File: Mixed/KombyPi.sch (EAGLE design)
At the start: 15 parts, among them IC3 DS1307, J1 POWER_JACKPTH, J2 MOLEX-39501XXX4, Q1 32.768

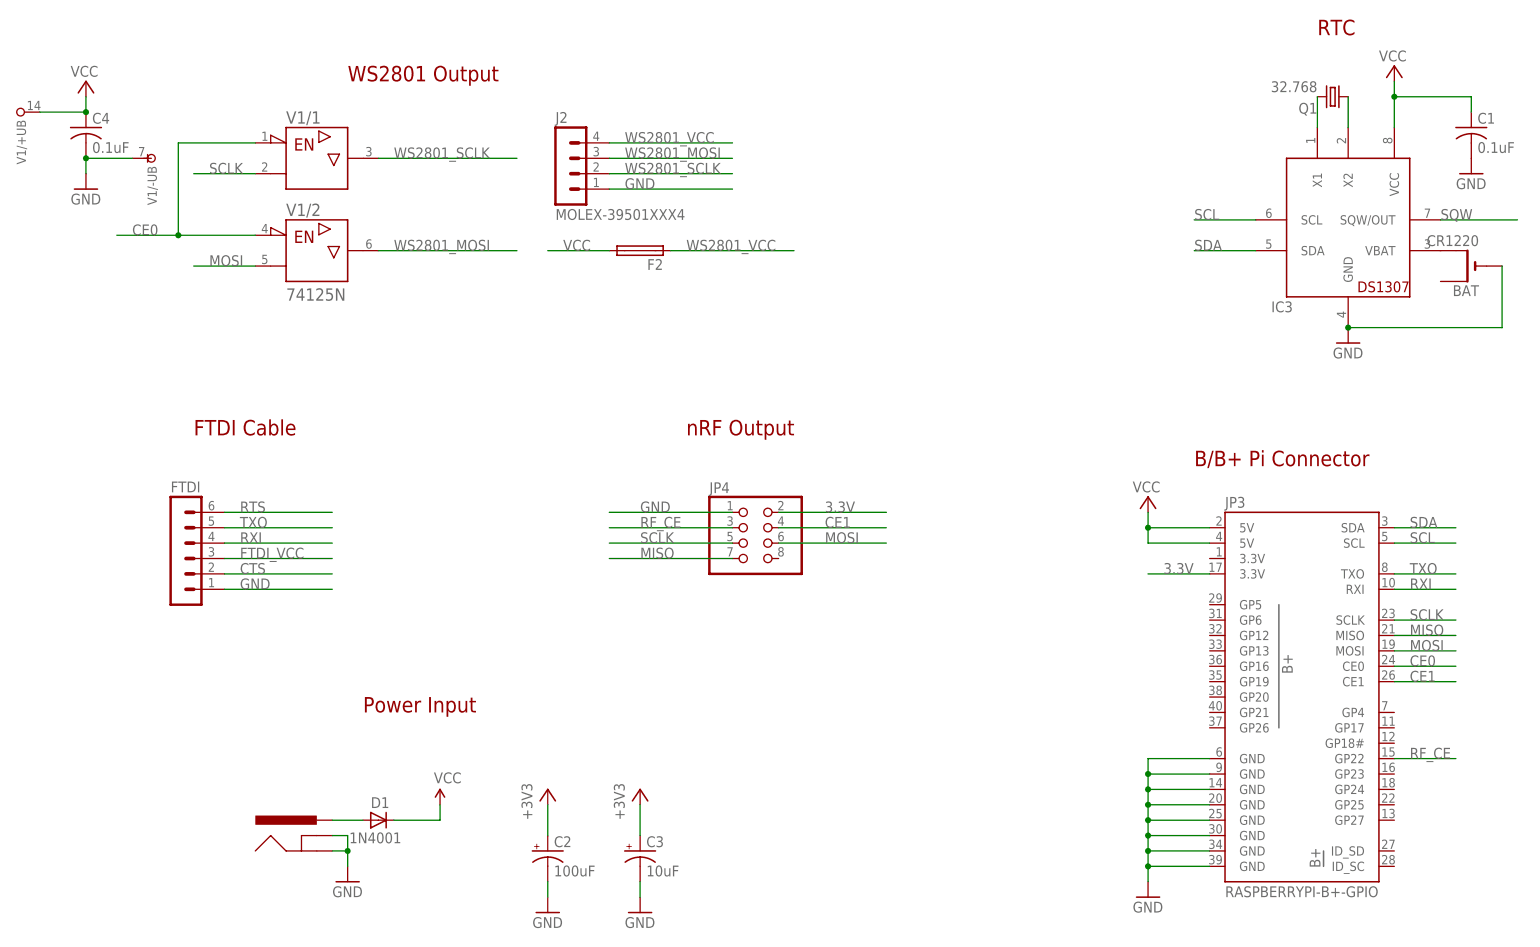
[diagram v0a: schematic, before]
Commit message: Update KombyPi mixed boards to be cleaner layout.
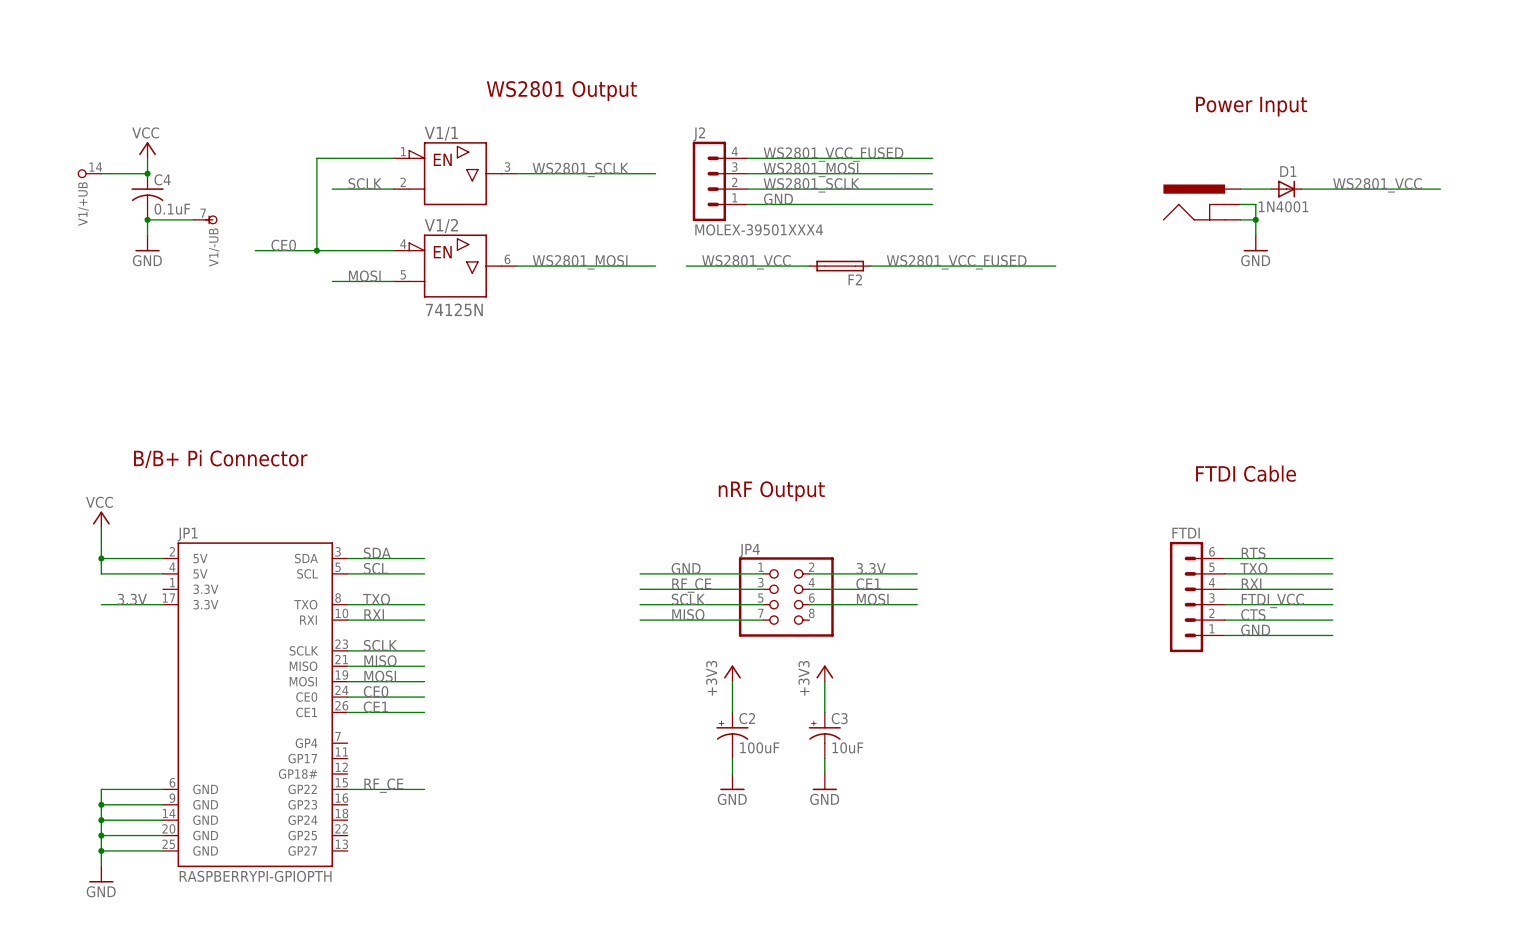
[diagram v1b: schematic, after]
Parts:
- removed BAT: CR1220, adafruit:CR1220THM
- removed C1: 0.1uF, adafruit:C-US025-025X050
- removed IC3: DS1307, adafruit:DS1307
- removed JP3: RASPBERRYPI-B+-GPIO, SparkFun-Boards:RASPBERRYPI-B+-GPIO
- removed Q1: 32.768, crystal:CRYTALTC38H
- added JP1: RASPBERRYPI-GPIOPTH, SparkFun-Boards:RASPBERRYPI-GPIOPTH
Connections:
- removed net N$14: IC3.X1, Q1.2
- removed net N$15: IC3.X2, Q1.1
- removed net N$39: BAT.+1, IC3.VBAT
- removed net SQW: IC3.SQW/OUT
- new net WS2801_VCC_FUSED: F2.1, J2.4
- net 3.3V: now also JP1.3.3V@17; no longer JP3.3.3V@17
- net CE0: now also JP1.CE0; no longer JP3.CE0
- net CE1: now also JP1.CE1; no longer JP3.CE1
- net GND: now also JP1.GND@14, JP1.GND@20, JP1.GND@25, JP1.GND@6, JP1.GND@9; no longer BAT.-, C1.2, IC3.GND, JP3.GND@14, JP3.GND@20, JP3.GND@25, JP3.GND@30, JP3.GND@34, JP3.GND@39, JP3.GND@6, JP3.GND@9
- net MISO: now also JP1.MISO; no longer JP3.MISO
- net MOSI: now also JP1.MOSI; no longer JP3.MOSI
- net RF_CE: now also JP1.GP22; no longer JP3.GP22
- net RXI: now also JP1.RXI; no longer JP3.RXI
- net SCL: now also JP1.SCL; no longer IC3.SCL, JP3.SCL
- net SCLK: now also JP1.SCLK; no longer JP3.SCLK
- net SDA: now also JP1.SDA; no longer IC3.SDA, JP3.SDA
- net TXO: now also JP1.TXO; no longer JP3.TXO
- net VCC: now also JP1.5V@2, JP1.5V@4; no longer C1.1, D1.C, F2.2, IC3.VCC, JP3.5V@2, JP3.5V@4
- net WS2801_VCC: now also D1.C, F2.2; no longer F2.1, J2.4
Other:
- note removed: "RTC"
- moved on the sheet: C2, C3, C4, D1, F2, FTDI, J2, JP4, V1/+UB, V1/-UB, V1/1, V1/2
